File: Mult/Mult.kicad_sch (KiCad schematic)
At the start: 55 parts, among them J1 Conn_02x05_Odd_Even, J10 AudioJack2_SwitchT, J11 AudioJack2_SwitchT, J12 AudioJack2_SwitchT, J13 AudioJack2_SwitchT, J14 AudioJack2_SwitchT, J15 AudioJack2_SwitchT, J2 AudioJack2_SwitchT, J3 AudioJack2_SwitchT, J4 AudioJack2_SwitchT, J5 AudioJack2_SwitchT, J6 AudioJack2_SwitchT, J7 AudioJack2_SwitchT, J8 AudioJack2_SwitchT, J9 AudioJack2_SwitchT, U1 TL072, U2 TL072, U3 TL072, U4 TL072, U5 TL072, U6 TL072

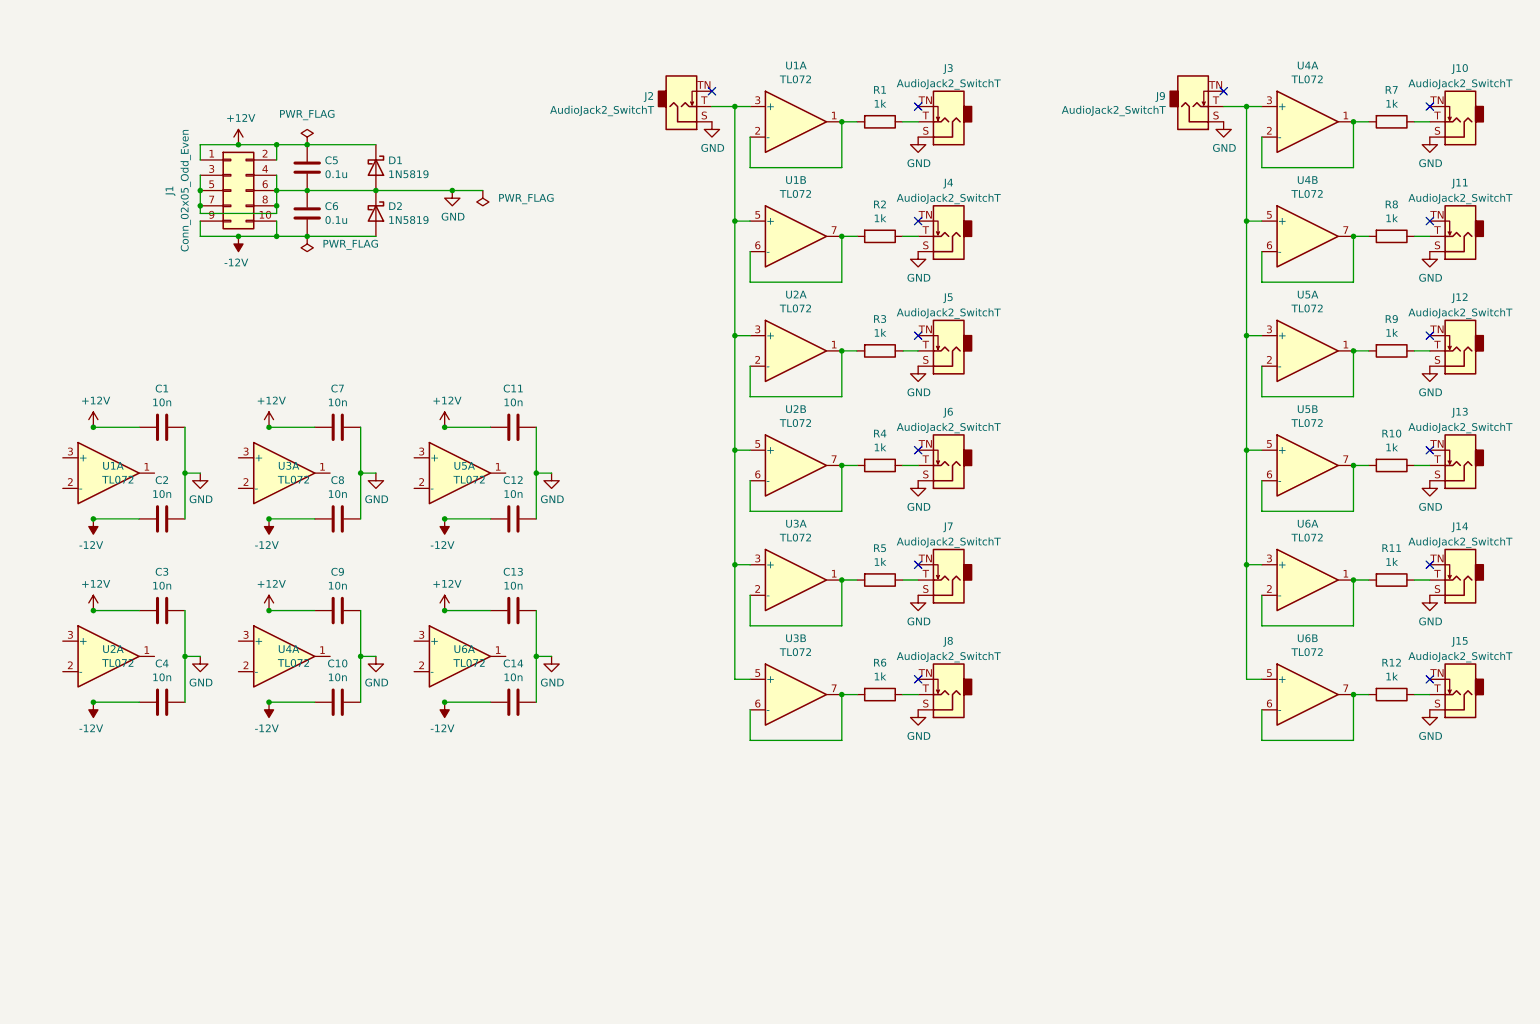
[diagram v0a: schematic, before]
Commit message: Finish main set of revisions
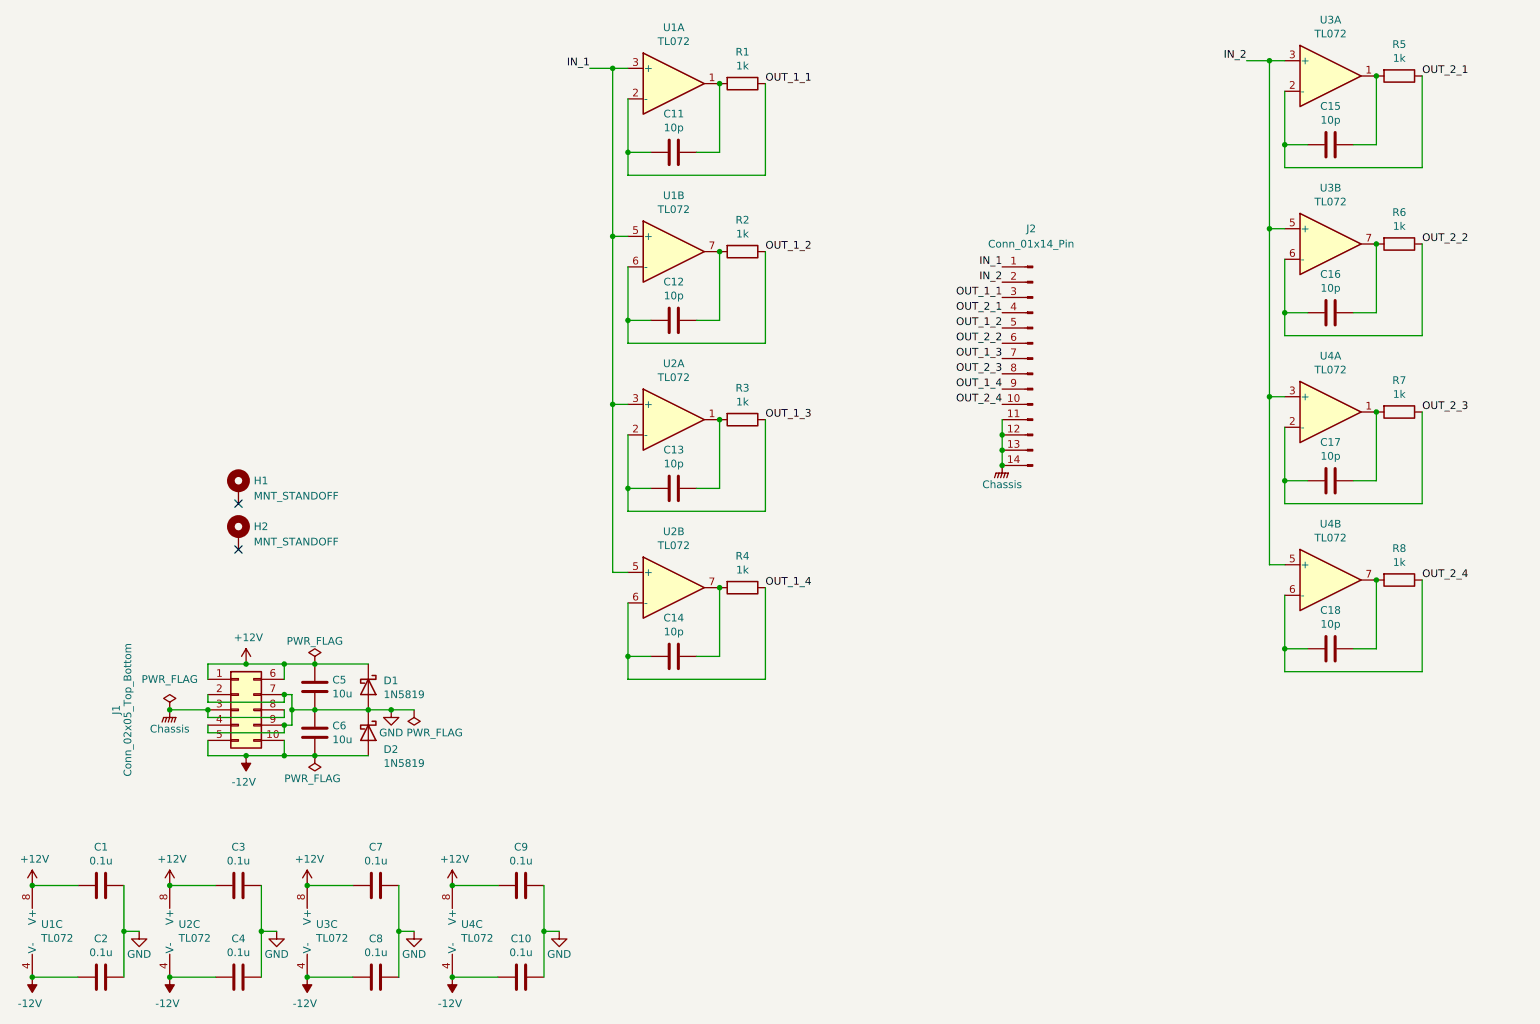
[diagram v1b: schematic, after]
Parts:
- removed J1: Conn_02x05_Odd_Even, Connector_PinHeader_2.54mm:PinHeader_2x05_P2.54mm_Vertical, symbol Connector_Generic:Conn_02x05_Odd_Even
- removed J10, J11, J12, J13, J14, J15, J2, J3, J4, J5, J6, J7, J8, J9: AudioJack2_SwitchT, Connector_Audio:Jack_3.5mm_QingPu_WQP-PJ398SM_Vertical_CircularHoles, symbol Connector:AudioJack2_SwitchT
- removed R10, R11, R12, R5, R9: 1k, Resistor_THT:R_Axial_DIN0207_L6.3mm_D2.5mm_P7.62mm_Horizontal, symbol Device:R
- removed unit 1 of U2 (x2)
- removed unit 1 of U3 (x2)
- removed U5 (x2), U6 (x2): TL072, Package_DIP:DIP-8_W7.62mm_Socket, symbol Amplifier_Operational:TL072
- added C15, C16, C17, C18: 10p, 0_Capacitor_THT:C_Disc_D5.5mm_W2.5mm_P2.50mm, symbol Device:C
- added H1, H2: MNT_STANDOFF, 0_MountingHole:MountingHole_Pitch7.5mm_Drill3.4mm, symbol Mechanical:MountingHole_Pad
- added J1: Conn_02x05_Top_Bottom, Connector_Molex:Molex_Mini-Fit_Jr_5566-10A_2x05_P4.20mm_Vertical, symbol Connector_Generic:Conn_02x05_Top_Bottom
- added J2: Conn_01x14_Pin, Connector_PinHeader_2.54mm:PinHeader_1x14_P2.54mm_Vertical, symbol Connector:Conn_01x14_Pin
- added R7: 1k, Resistor_THT:R_Axial_DIN0207_L6.3mm_D2.5mm_P7.62mm_Horizontal, symbol Device:R
- added unit 3 of U2
- added unit 1 of U2
- added unit 3 of U3
- added unit 3 of U4
- C1, C10, C2, C3, C4, C7, C8, C9: value 10n -> 0.1u; footprint Capacitor_THT:C_Disc_D5.0mm_W2.5mm_P5.00mm -> 0_Capacitor_THT:C_Disc_D5.5mm_W2.5mm_P2.50mm
- C11, C12, C13, C14: value 10n -> 10p; footprint Capacitor_THT:C_Disc_D5.0mm_W2.5mm_P5.00mm -> 0_Capacitor_THT:C_Disc_D5.5mm_W2.5mm_P2.50mm
- C5, C6: value 0.1u -> 10u; footprint Capacitor_THT:C_Disc_D5.0mm_W2.5mm_P5.00mm -> 0_Capacitor_THT:C_Disc_D5.5mm_W4.0mm_P2.50mm
- renumbered R7 to R5, U4 to U3
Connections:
- net +12V: now also U1.8 (V+), J1.1 (Pin_1), J1.6 (Pin_6), U2.8 (V+), U3.8 (V+), U4.8 (V+); no longer C11.1, C13.1
- net -12V: now also U1.4 (V-), J1.10 (Pin_10), J1.5 (Pin_5), U2.4 (V-), U3.4 (V-), U4.4 (V-); no longer C12.1, C14.1
- net GND: now also J1.2 (Pin_2), J1.4 (Pin_4), J1.7 (Pin_7), J1.9 (Pin_9); no longer C11.2, C12.2, C13.2, C14.2
- net at R1.2, U1.1: now also C11.2; no longer U1.2 (-)
- net IN_1: now reaches U1.3 (+), U1.5 (+), U2.5 (+)
- net IN_1: now also J2.1 (Pin_1), U2.3 (+); no longer U3.5 (+)
- net OUT_1_1: now reaches R1.1
- net OUT_1_1: now also C11.1, U1.2 (-), J2.3 (Pin_3)
- net at R2.2, U1.7: now also C12.2; no longer U1.6 (-)
- net OUT_1_2: now reaches R2.1
- net OUT_1_2: now also C12.1, U1.6 (-), J2.5 (Pin_5)
- net at R3.2: now also C13.2, U2.1
- net OUT_1_3: now reaches R3.1
- net OUT_1_3: now also C13.1, J2.7 (Pin_7), U2.2 (-)
- net at R4.2, U2.7: now also C14.2; no longer U2.6 (-)
- net OUT_1_4: now reaches R4.1
- net OUT_1_4: now also C14.1, U2.6 (-), J2.9 (Pin_9)
- net at R6.2, U3.7: now also C16.2; no longer U3.6 (-)
- net OUT_2_2: now reaches R6.1
- net OUT_2_2: now also U3.6 (-), C16.1, J2.6 (Pin_6)
- net at R5.2, U3.1: now also C15.2; no longer U3.2 (-)
- net IN_2: now reaches U3.3 (+), U4.5 (+)
- net IN_2: now also U3.5 (+), U4.3 (+), J2.2 (Pin_2)
- net OUT_2_1: now reaches R5.1
- net OUT_2_1: now also U3.2 (-), C15.1, J2.4 (Pin_4)
- net at R8.2, U4.7: now also C18.2; no longer U4.6 (-)
- net OUT_2_4: now reaches R8.1
- net OUT_2_4: now also U4.6 (-), C18.1, J2.10 (Pin_10)
- net at U4.1: now also C17.2, R7.2
- net OUT_2_3: now reaches U4.2 (-)
- net OUT_2_3: now also C17.1, J2.8 (Pin_8), R7.1
- new net Chassis: J1.3 (Pin_3), J1.8 (Pin_8), J2.11 (Pin_11), J2.12 (Pin_12), J2.13 (Pin_13), J2.14 (Pin_14)
- no-connect marks 14 -> 2
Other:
- moved on the sheet: C1, C2, R5, U3A
